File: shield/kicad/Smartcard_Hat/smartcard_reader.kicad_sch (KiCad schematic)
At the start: 26 parts, among them J8 7712P0225A25LF, U1 ST8034HNQR

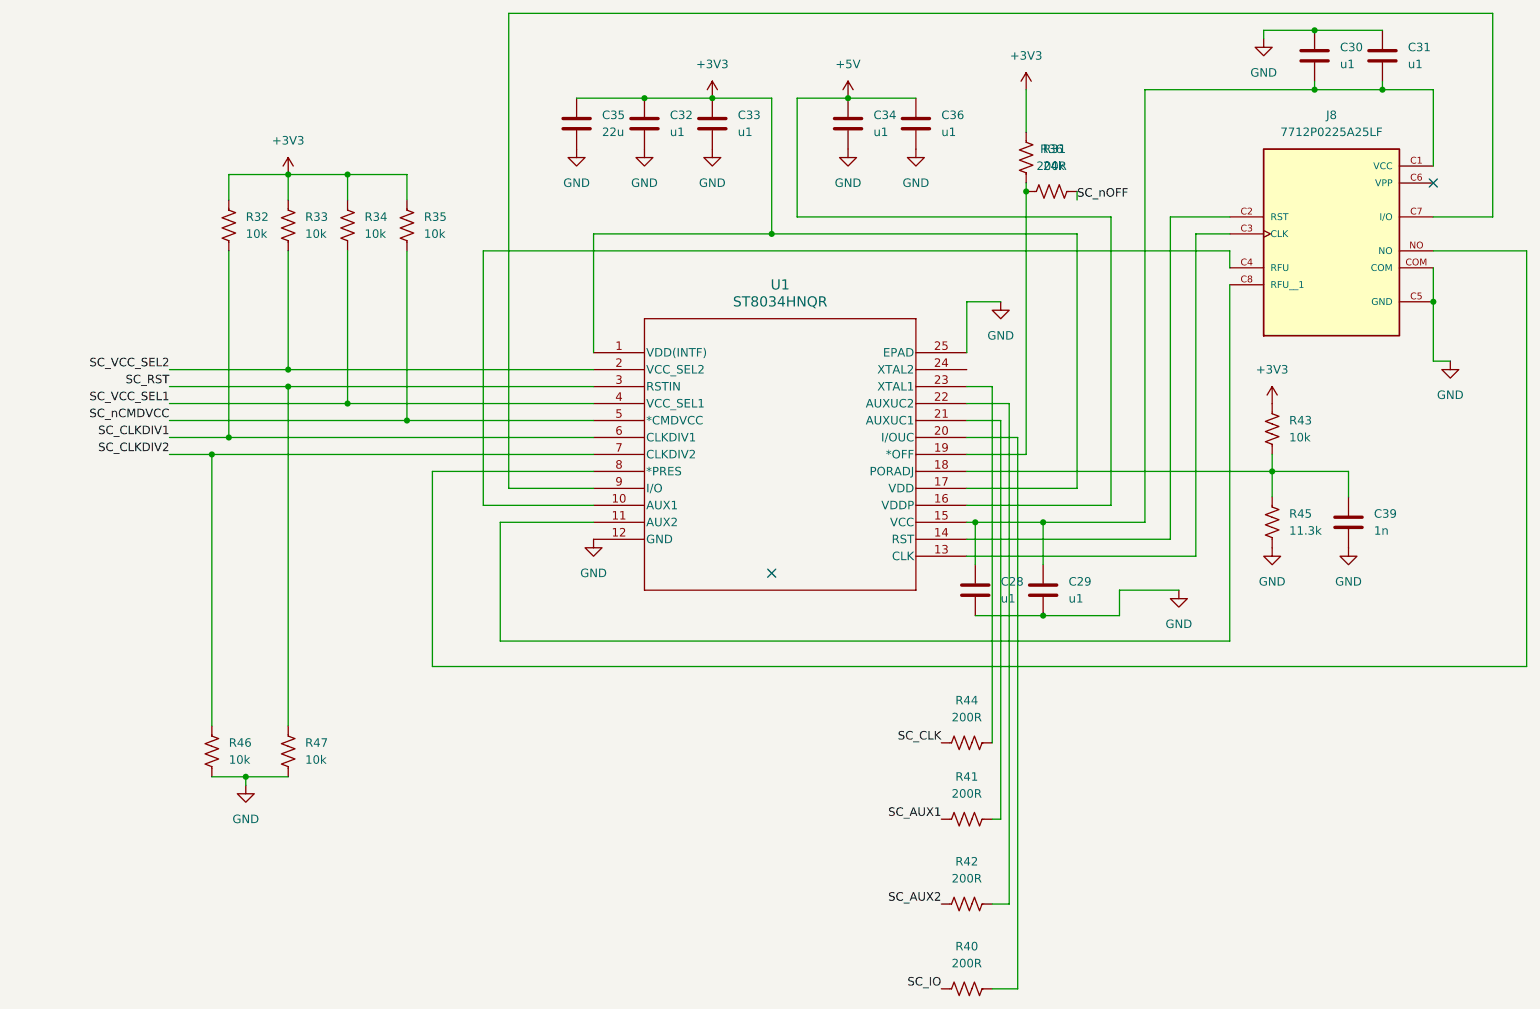
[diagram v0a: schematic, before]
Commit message: wip
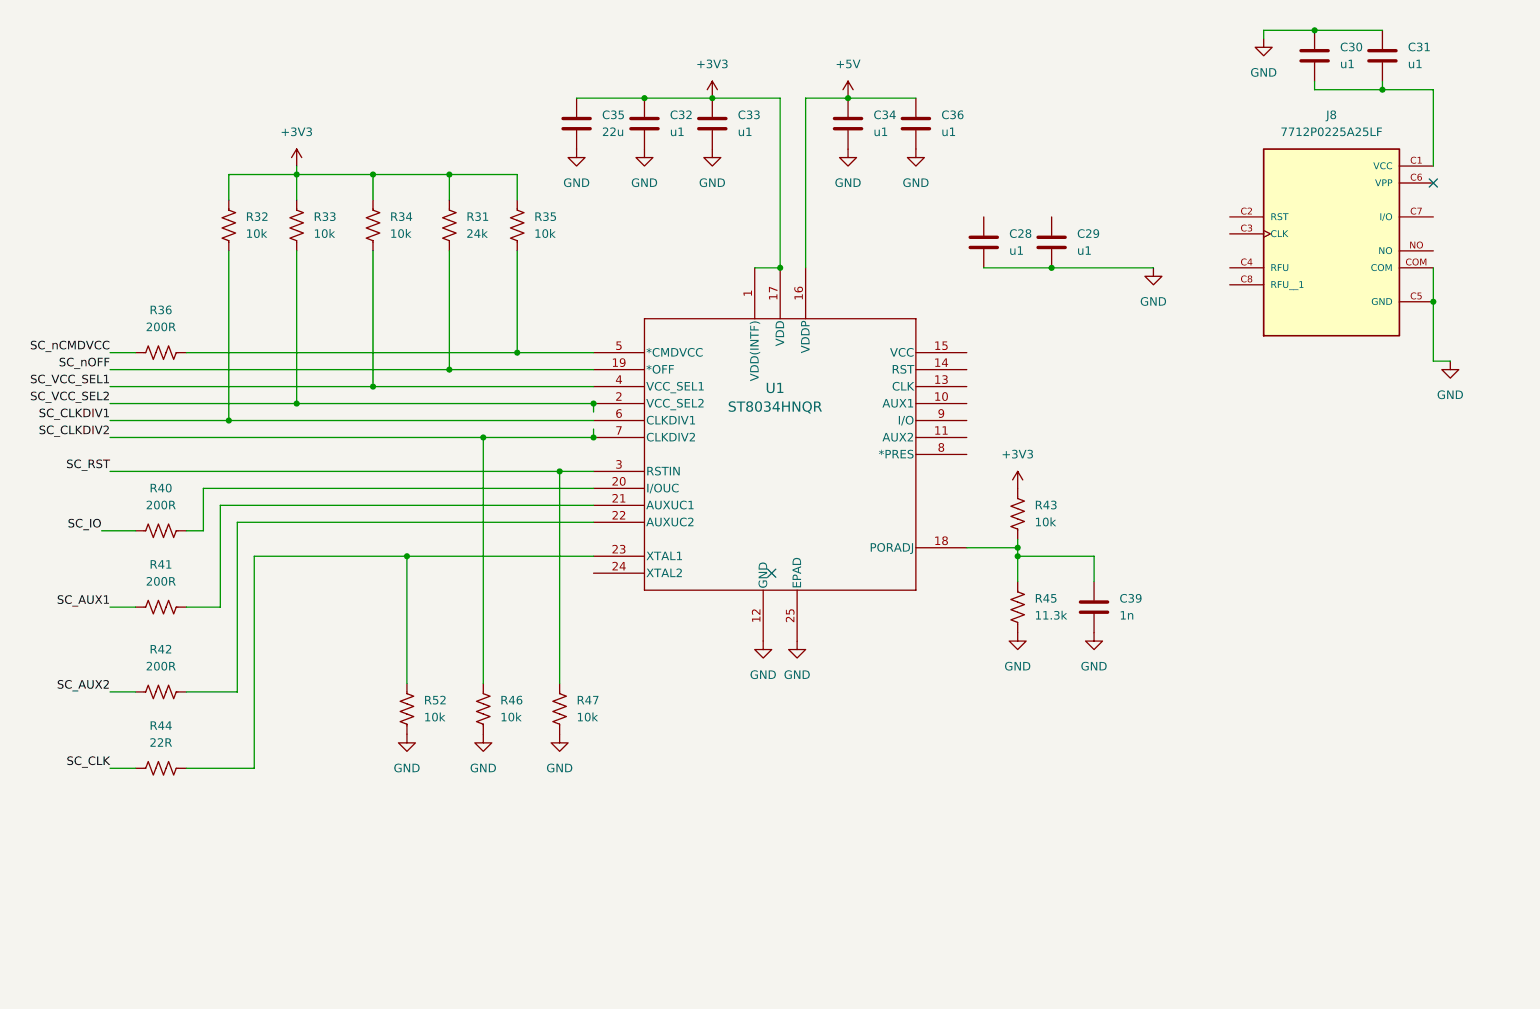
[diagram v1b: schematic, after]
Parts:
- added R52: 10k, Resistor_SMD:R_0402_1005Metric_Pad0.72x0.64mm_HandSolder, symbol Device:R_US
- R44: value 200R -> 22R
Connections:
- net GND: now also R52.2
- net SC_nCMDVCC: now also R36.1; no longer R35.2, U1.5 (*CMDVCC)
- net SC_nOFF: now also R31.2, U1.19 (*OFF); no longer R36.2
- net at C30.2, C31.2, J8.C1 (VCC): no longer C28.1, C29.1, U1.15 (VCC)
- net at R44.2, U1.23 (XTAL1): now also R52.1
- net at J8.C2 (RST): no longer U1.14 (RST)
- net at J8.C3 (CLK): no longer U1.13 (CLK)
- net at J8.C4 (RFU): no longer U1.10 (AUX1)
- net at J8.C7 (I/O): no longer U1.9 (I/O)
- net at J8.C8 (RFU__1): no longer U1.11 (AUX2)
- net at J8.NO: no longer U1.8 (*PRES)
- new net: R35.2, R36.2, U1.5 (*CMDVCC)
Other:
- moved on the sheet: C28, C29, C39, R31, R33, R34, R35, R36, R40, R41, R42, R43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
